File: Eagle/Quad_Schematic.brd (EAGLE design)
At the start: 100 x 80 mm, 36 parts, among them J1 FTDI_DEVICE, M1 WIRELESS-NRF24L01, U1 ATMEGA328P_TQFP, U2 GY-521MPU6050

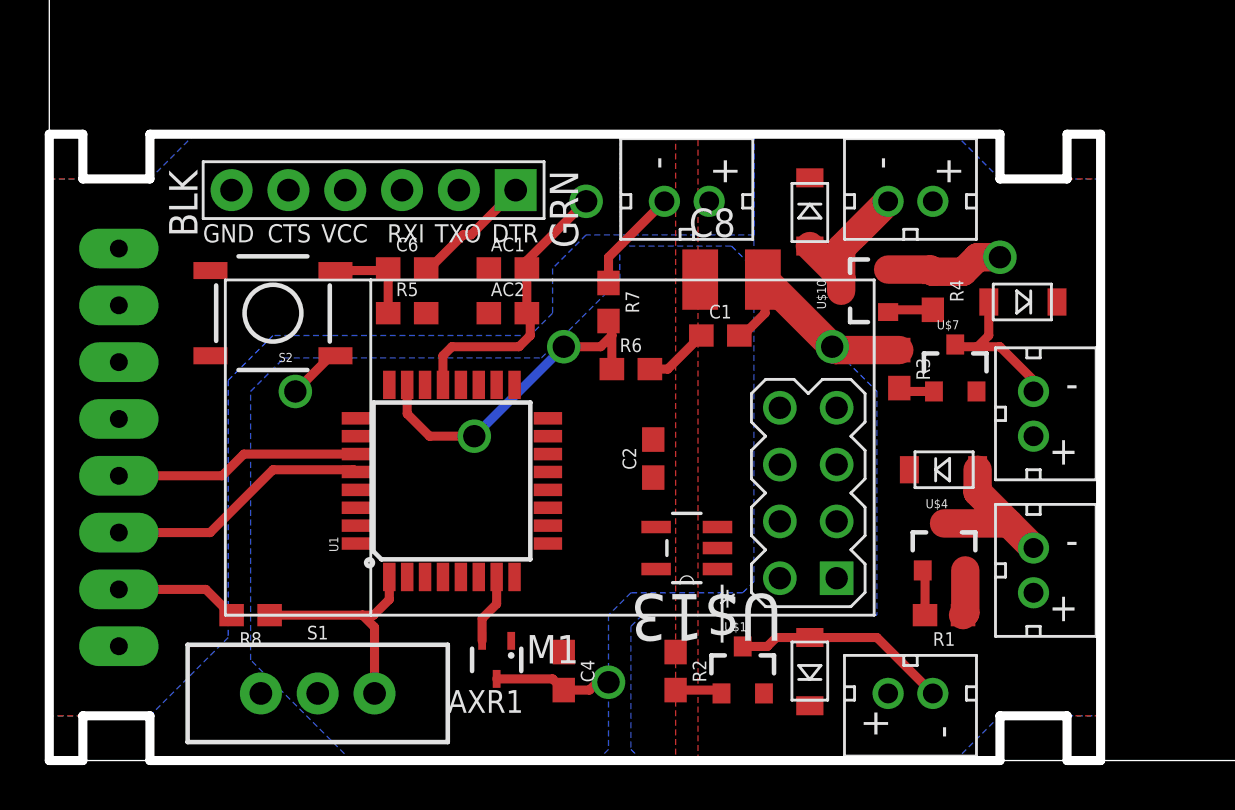
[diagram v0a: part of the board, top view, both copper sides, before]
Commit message: the first submission
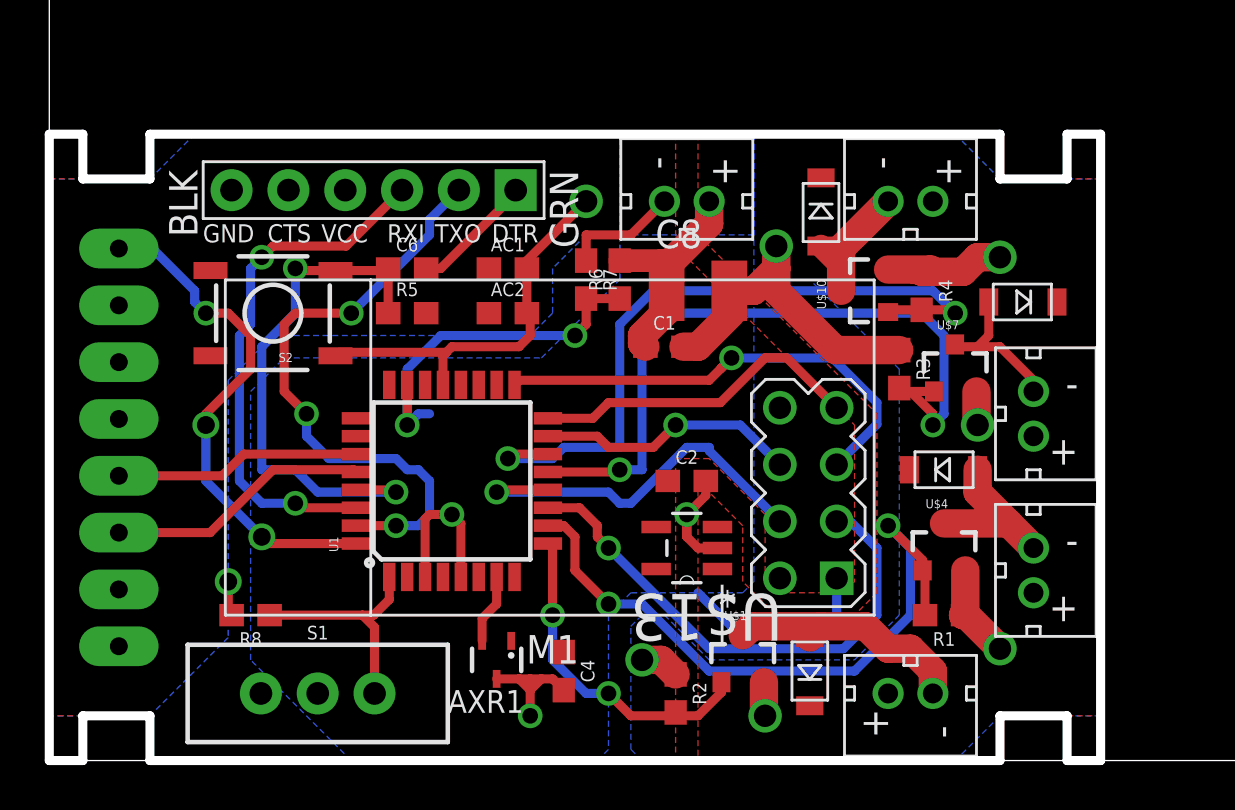
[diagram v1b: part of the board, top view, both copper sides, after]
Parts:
- moved R6 4.03 mm to (25.5, 21.5), turned to 90 degrees
- moved C1 2.55 mm to (27.5, 18.5)
- moved C2 1.80 mm to (28.5, 12.5), turned to 0 degrees
- moved C8 1.58 mm to (29.0, 21.0)
- moved R7 1.41 mm to (24.0, 21.5)
- moved R2 1.00 mm to (28.0, 3.00)
- moved R4 0.50 mm to (39.0, 21.0)
- moved U$1 0.50 mm to (31.0, 4.50)
- moved U$12 0.50 mm to (34.5, 24.5)
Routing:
- net GND: track 48.5 -> 82.3 mm, vias 5 -> 11
- net M3: track 1.61 -> 32.3 mm, vias 0 -> 2
- net M4: track 2.04 -> 31.7 mm, vias 0 -> 2
- net M2: track 2.04 -> 29.9 mm, vias 0 -> 2
- net TX0: track 0.00 -> 27.4 mm, vias 0 -> 3
- net RXI: track 0.00 -> 23.9 mm, vias 0 -> 2
- net CE: track 0.00 -> 23.5 mm, vias 0 -> 1
- net INT: track 0.00 -> 23.0 mm, vias 0 -> 3
- net SCK: track 0.00 -> 21.8 mm, vias 0 -> 1
- net RESET: track 4.40 -> 24.1 mm, vias 0 -> 2
- net CS: track 0.00 -> 18.1 mm, vias 0 -> 1
- net MISO: track 0.00 -> 14.9 mm
- net M1: track 2.11 -> 14.9 mm, vias 0 -> 2
- net MOSI: track 0.00 -> 11.7 mm, vias 0 -> 1
- net MVCC: track 2.92 -> 10.0 mm
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
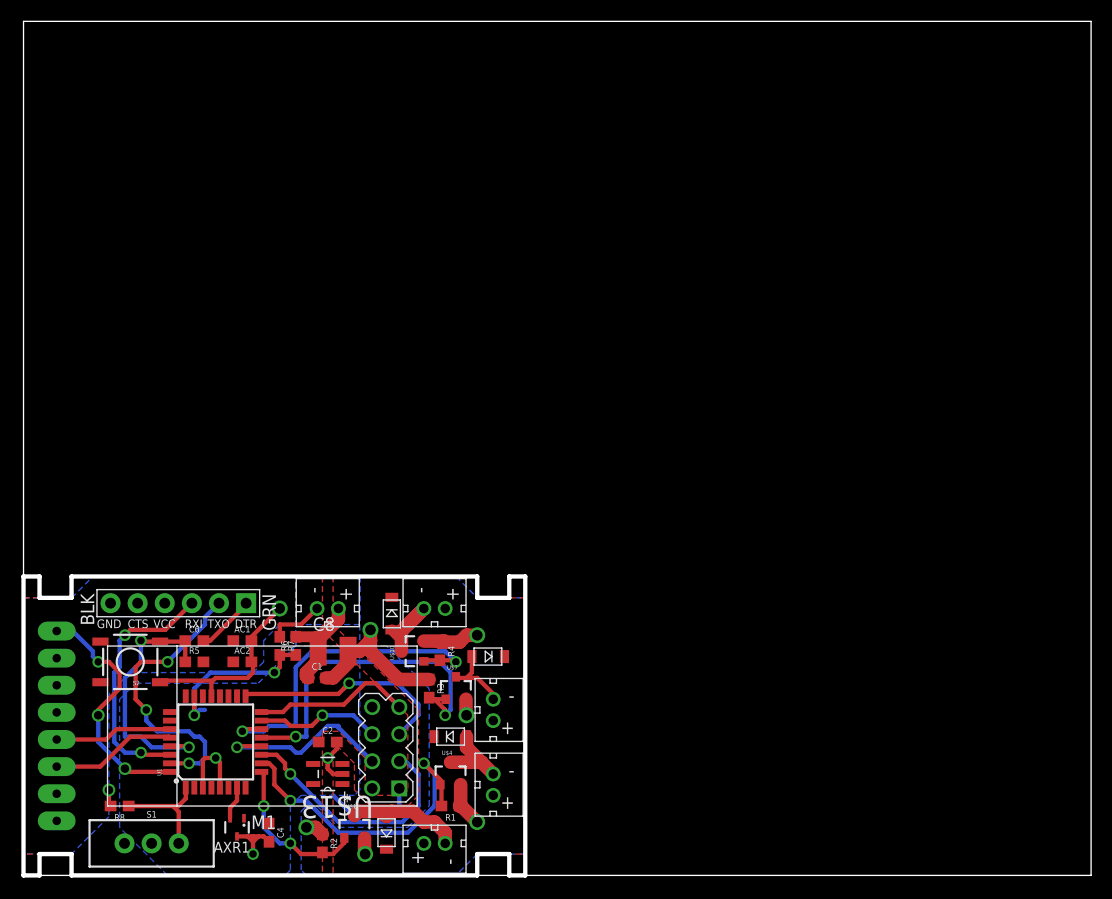
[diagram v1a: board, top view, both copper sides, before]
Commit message: 2 airwires left
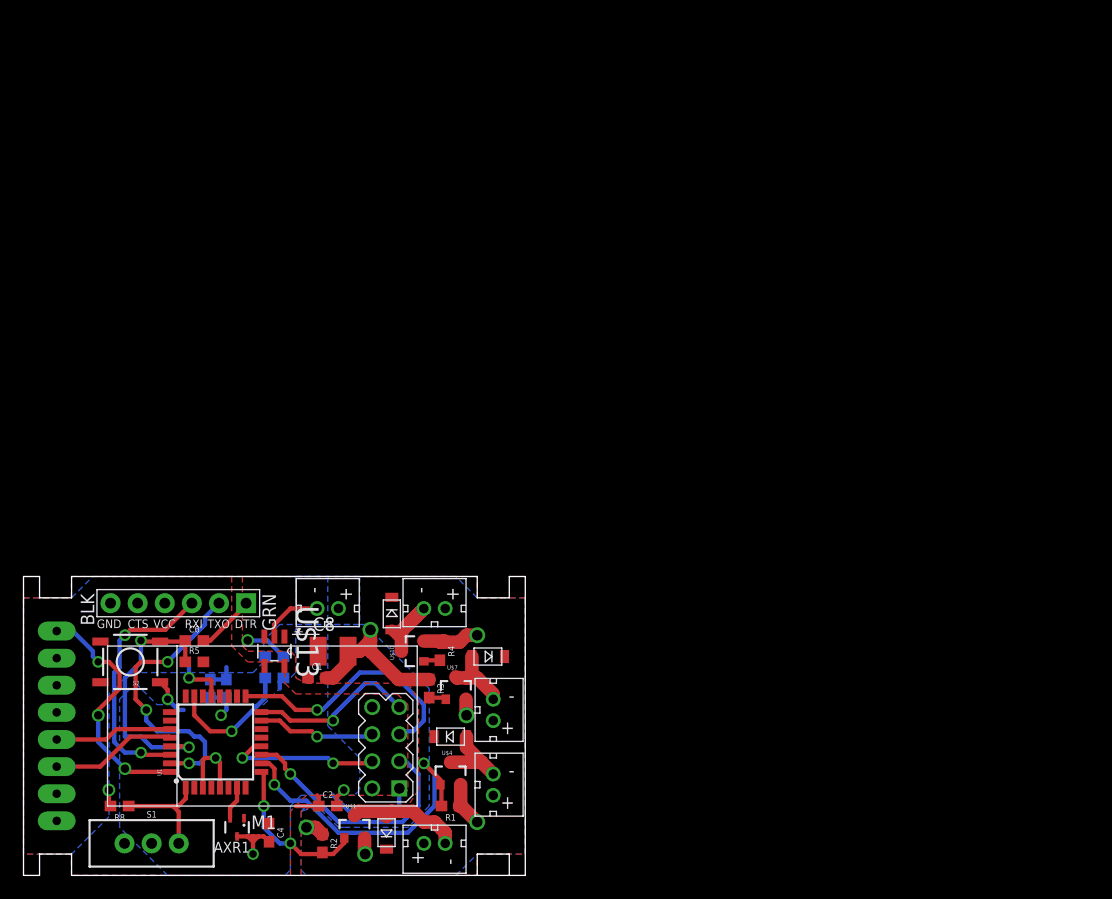
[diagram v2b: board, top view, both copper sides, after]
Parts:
- moved U$13 12.5 mm to (23.5, 21.0), turned to 270 degrees
- moved C2 6.00 mm to (28.5, 6.50)
- moved AC1 4.74 mm to (19.0, 17.5), flipped to the bottom, turned to 90 degrees
- moved AC2 3.91 mm to (17.5, 17.5), flipped to the bottom, turned to 90 degrees
- moved R7 3.04 mm to (23.5, 18.5), flipped to the bottom, turned to 0 degrees
- moved R6 2.24 mm to (23.5, 20.5), flipped to the bottom, turned to 180 degrees
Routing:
- net M3: track 32.3 -> 1.61 mm, vias 2 -> 0
- net M4: track 31.7 -> 1.54 mm, vias 2 -> 0
- net GND: track 82.3 -> 73.6 mm, vias 11 -> 12
- net 3V3: track 0.00 -> 6.57 mm, vias 0 -> 1
- net MVCC: track 10.0 -> 3.97 mm, vias 0 -> 1
- net CS: track 18.1 -> 15.1 mm, vias 1 -> 2
- net BATT_CHECK: track 17.0 -> 14.2 mm, vias 2 -> 1
- net SCK: track 21.8 -> 24.3 mm
- net MISO: track 14.9 -> 16.2 mm, vias 0 -> 1
- net MOSI: track 11.7 -> 11.1 mm
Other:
- board size 100 x 80 mm -> 47 x 28 mm
